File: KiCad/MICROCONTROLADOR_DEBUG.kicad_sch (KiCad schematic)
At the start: 9 parts, among them U7 PIC24HJ128GP504-I_PT, Y1 8MHz

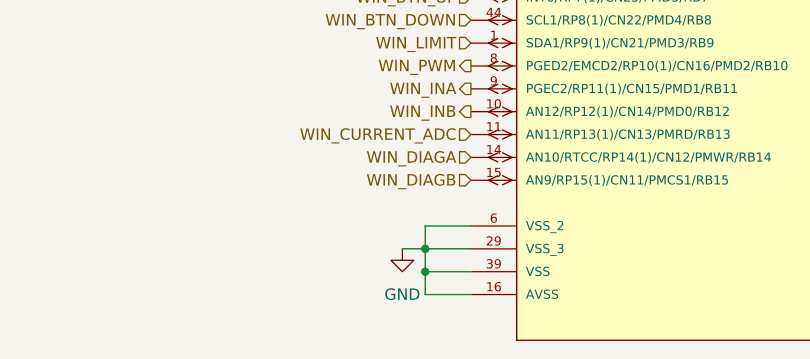
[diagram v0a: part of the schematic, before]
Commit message: Versió final de l'esquematic
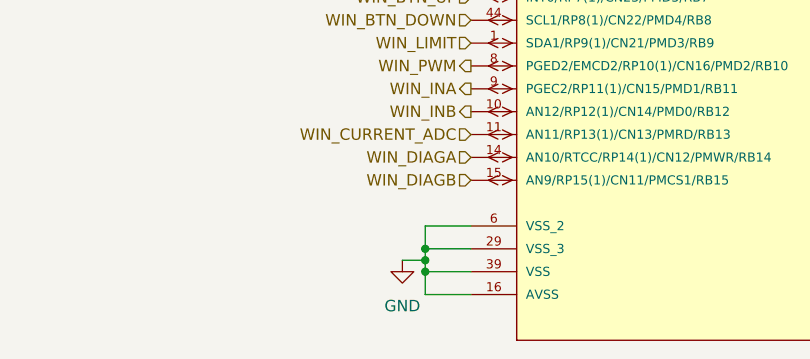
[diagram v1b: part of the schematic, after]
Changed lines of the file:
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@@
+		(color 0 0 0 0)
+	)
+	(junction
+		(at 88.9 130.81)
+		(diameter 0)
 		(color 0 0 0 0)
 	)
@@
 	(wire
 		(pts
+			(xy 88.9 129.54) (xy 88.9 130.81)
+		)
+		(stroke
+			(width 0)
+			(type default)
+		)
+	)
+	(wire
+		(pts
+			(xy 87.63 33.02) (xy 87.63 35.56)
+		)
+		(stroke
+			(width 0)
+			(type default)
+		)
+	)
+	(wire
+		(pts
+			(xy 53.34 27.94) (xy 58.42 27.94)
+		)
+		(stroke
+			(width 0)
+			(type default)
+		)
+	)
+	(wire
+		(pts
+			(xy 87.63 33.02) (xy 93.98 33.02)
+		)
+		(stroke
+			(width 0)
+			(type default)
+		)
+	)
+	(wire
+		(pts
+			(xy 77.47 38.1) (xy 77.47 35.56)
+		)
+		(stroke
+			(width 0)
+			(type default)
+		)
+	)
+	(wire
+		(pts
+			(xy 60.96 74.93) (xy 64.77 74.93)
+		)
+		(stroke
+			(width 0)
+			(type default)
+		)
+	)
+	(wire
+		(pts
+			(xy 67.31 27.94) (xy 77.47 27.94)
+		)
+		(stroke
+			(width 0)
+			(type default)
+		)
+	)
+	(wire
+		(pts
+			(xy 48.26 74.93) (xy 48.26 77.47)
+		)
+		(stroke
+			(width 0)
+			(type default)
+		)
+	)
+	(wire
+		(pts
+			(xy 93.98 134.62) (xy 88.9 134.62)
+		)
+		(stroke
+			(width 0)
+			(type default)
+		)
+	)
+	(wire
+		(pts
+			(xy 68.58 45.72) (xy 93.98 45.72)
+		)
+		(stroke
+			(width 0)
+			(type default)
+		)
+	)
+	(wire
+		(pts
+			(xy 50.8 27.94) (xy 53.34 27.94)
+		)
+		(stroke
+			(width 0)
+			(type default)
+		)
+	)
+	(wire
+		(pts
 			(xy 88.9 132.08) (xy 93.98 132.08)
 		)
@@
 	(wire
 		(pts
-			(xy 88.9 129.54) (xy 88.9 132.08)
-		)
-		(stroke
-			(width 0)
-			(type default)
-		)
-	)
-	(wire
-		(pts
-			(xy 87.63 33.02) (xy 87.63 35.56)
-		)
-		(stroke
-			(width 0)
-			(type default)
-		)
-	)
-	(wire
-		(pts
-			(xy 53.34 27.94) (xy 58.42 27.94)
-		)
-		(stroke
-			(width 0)
-			(type default)
-		)
-	)
-	(wire
-		(pts
-			(xy 87.63 33.02) (xy 93.98 33.02)
-		)
-		(stroke
-			(width 0)
-			(type default)
-		)
-	)
-	(wire
-		(pts
-			(xy 88.9 134.62) (xy 88.9 132.08)
-		)
-		(stroke
-			(width 0)
-			(type default)
-		)
-	)
-	(wire
-		(pts
-			(xy 77.47 38.1) (xy 77.47 35.56)
-		)
-		(stroke
-			(width 0)
-			(type default)
-		)
-	)
-	(wire
-		(pts
-			(xy 60.96 74.93) (xy 64.77 74.93)
-		)
-		(stroke
-			(width 0)
-			(type default)
-		)
-	)
-	(wire
-		(pts
-			(xy 67.31 27.94) (xy 77.47 27.94)
-		)
-		(stroke
-			(width 0)
-			(type default)
-		)
-	)
-	(wire
-		(pts
-			(xy 86.36 129.54) (xy 88.9 129.54)
-		)
-		(stroke
-			(width 0)
-			(type default)
-		)
-	)
-	(wire
-		(pts
-			(xy 48.26 74.93) (xy 48.26 77.47)
-		)
-		(stroke
-			(width 0)
-			(type default)
-		)
-	)
-	(wire
-		(pts
-			(xy 93.98 134.62) (xy 88.9 134.62)
-		)
-		(stroke
-			(width 0)
-			(type default)
-		)
-	)
-	(wire
-		(pts
-			(xy 68.58 45.72) (xy 93.98 45.72)
-		)
-		(stroke
-			(width 0)
-			(type default)
-		)
-	)
-	(wire
-		(pts
-			(xy 50.8 27.94) (xy 53.34 27.94)
-		)
-		(stroke
-			(width 0)
-			(type default)
-		)
-	)
-	(wire
-		(pts
 			(xy 48.26 63.5) (xy 48.26 74.93)
 		)
@@
 	(wire
 		(pts
+			(xy 88.9 130.81) (xy 88.9 132.08)
+		)
+		(stroke
+			(width 0)
+			(type default)
+		)
+	)
+	(wire
+		(pts
 			(xy 64.77 66.04) (xy 64.77 74.93)
 		)
@@
 	(wire
 		(pts
+			(xy 86.36 130.81) (xy 88.9 130.81)
+		)
+		(stroke
+			(width 0)
+			(type default)
+		)
+	)
+	(wire
+		(pts
 			(xy 93.98 66.04) (xy 64.77 66.04)
 		)
@@
 		(pts
 			(xy 92.71 35.56) (xy 92.71 43.18)
+		)
+		(stroke
+			(width 0)
+			(type default)
+		)
+	)
+	(wire
+		(pts
+			(xy 88.9 132.08) (xy 88.9 134.62)
 		)
 		(stroke
@@
 	(symbol
 		(lib_id "power:GND")
-		(at 86.36 129.54 0)
+		(at 86.36 130.81 0)
 		(unit 1)
 		(exclude_from_sim no)
@@
 		(fields_autoplaced yes)
 		(property "Reference" "#PWR045"
+			(at 86.36 137.16 0)
+			(effects
+				(font
+					(size 1.27 1.27)
+				)
+				(hide yes)
+			)
+		)
+		(property "Value" "GND"
 			(at 86.36 135.89 0)
 			(effects
@@
 					(size 1.27 1.27)
 				)
-				(hide yes)
-			)
-		)
-		(property "Value" "GND"
-			(at 86.36 134.62 0)
-			(effects
-				(font
-					(size 1.27 1.27)
-				)
 			)
 		)
 		(property "Footprint" ""
-			(at 86.36 129.54 0)
+			(at 86.36 130.81 0)
 			(effects
 				(font
@@
 		)
 		(property "Datasheet" ""
-			(at 86.36 129.54 0)
+			(at 86.36 130.81 0)
 			(effects
 				(font
@@
 		)
 		(property "Description" "Power symbol creates a global label with name \"GND\" , ground"
-			(at 86.36 129.54 0)
-			(effects
-				(font
+			(at 86.36 130.81 0)
+			(effects
+				(font

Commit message: 1ra versióPCB
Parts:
- Y1: footprint Crystal:Crystal_HC49-U_Horizontal -> Crystal:Crystal_SMD_3225-4Pin_3.2x2.5mm
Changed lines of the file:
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@@
 			)
 		)
-		(property "Footprint" "Crystal:Crystal_HC49-U_Horizontal"
+		(property "Footprint" "Crystal:Crystal_SMD_3225-4Pin_3.2x2.5mm"
 			(at 57.15 74.93 0)
 			(effects
